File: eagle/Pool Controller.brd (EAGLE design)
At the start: 67.3 x 64.4 mm, 27 parts, among them J1 POWER_JACKPTH, J2 Temp_Pool, J3 Relay, J4 Solar_Mon, J5 Temp_Solar

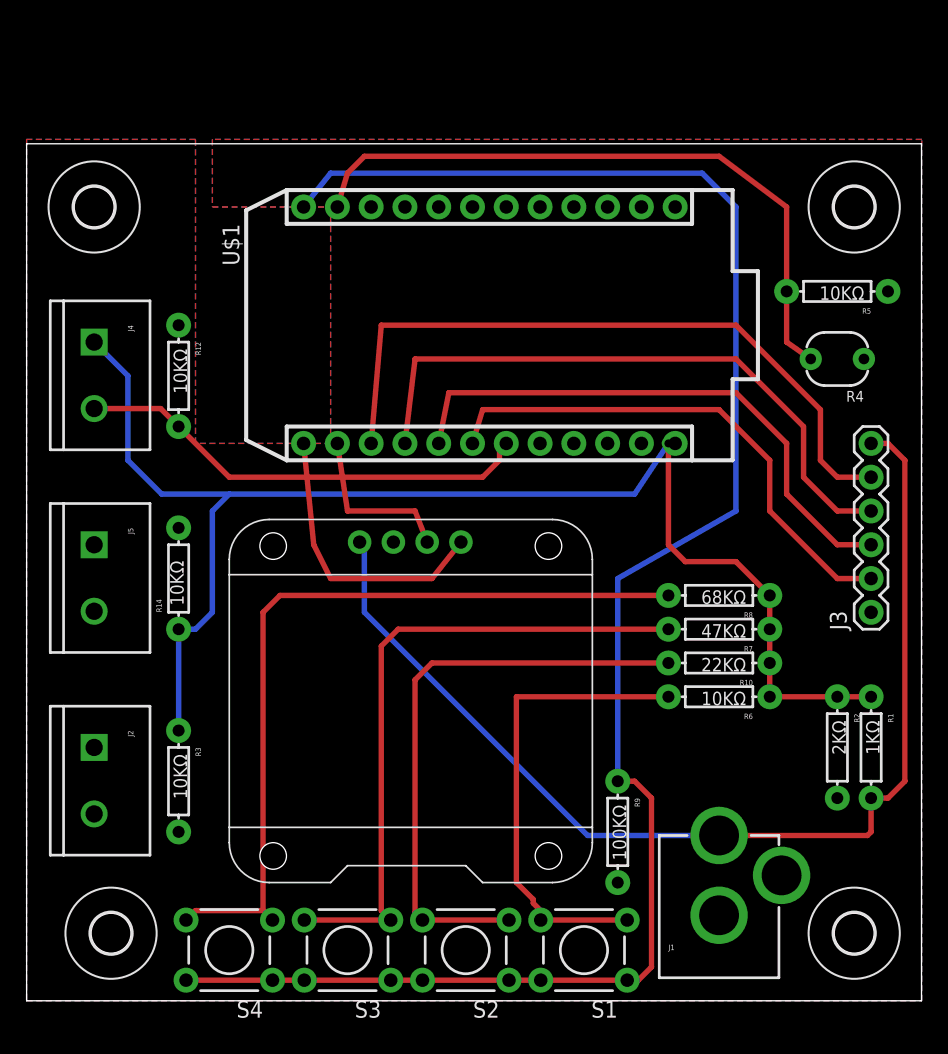
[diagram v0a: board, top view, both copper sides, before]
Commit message: Finished initial design
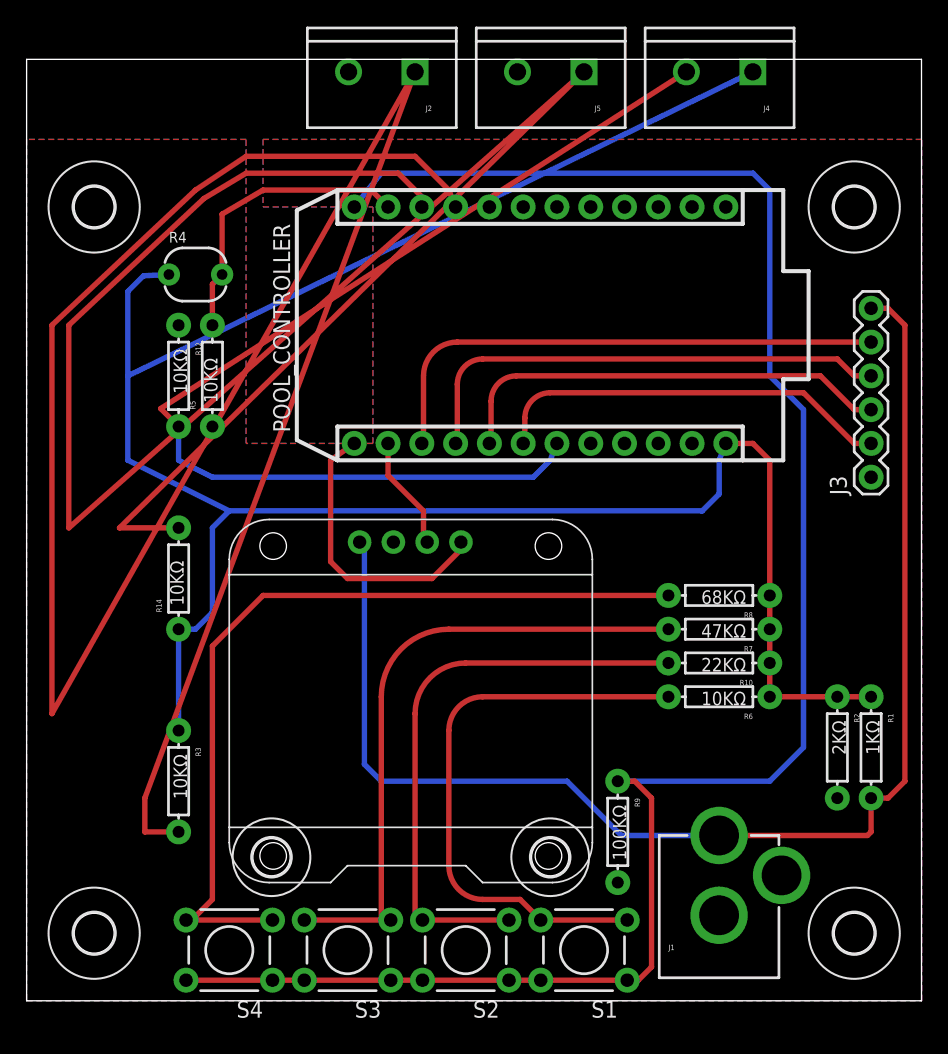
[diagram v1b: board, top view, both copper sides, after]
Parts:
- added POOL_CONTROLLER: PHOTON_WITH_HEADERS, Spark:PHOTON
- added U$7: (no value), holes:2,8
- U$1: value PHOTON_WITH_HEADERS -> (none); device Spark:PHOTON -> holes:2,8
- moved J2 56.2 mm to (27.9, 69.8), turned to 180 degrees
- moved J4 53.5 mm to (53.3, 69.8), turned to 180 degrees
- moved J5 51.2 mm to (40.6, 69.8), turned to 180 degrees
- moved U$1 50.2 mm to (17.1, 10.8), turned to 0 degrees
- moved R4 48.7 mm to (11.4, 54.6), turned to 0 degrees
- moved R5 47.4 mm to (12.7, 47.0), turned to 90 degrees
- moved J3 10.2 mm to (62.2, 39.4)
- moved U$4 1.27 mm to (3.81, 5.08)
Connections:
- removed net VCC: R4.1
- net 3.3V: now also POOL_CONTROLLER.24, R4.1; no longer U$1.24
- net GND: now also POOL_CONTROLLER.2, POOL_CONTROLLER.21; no longer U$1.2, U$1.21
- net N$1: now also POOL_CONTROLLER.15; no longer U$1.15
- net N$11: now also POOL_CONTROLLER.10; no longer U$1.10
- net N$12: now also POOL_CONTROLLER.9; no longer U$1.9
- net N$14: now also POOL_CONTROLLER.12; no longer U$1.12
- net N$2: now also POOL_CONTROLLER.16; no longer U$1.16
- net N$3: now also POOL_CONTROLLER.13; no longer U$1.13
- net N$4: now also POOL_CONTROLLER.14; no longer U$1.14
- net N$5: now also POOL_CONTROLLER.11; no longer U$1.11
- net N$6: now also POOL_CONTROLLER.17; no longer U$1.17
- net N$7: now also POOL_CONTROLLER.18; no longer U$1.18
- net N$9: now also POOL_CONTROLLER.19; no longer U$1.19
- net VBAT: now also POOL_CONTROLLER.22; no longer U$1.22
- net VIN: now also POOL_CONTROLLER.1; no longer U$1.1
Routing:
- net N$12: track 0.00 -> 185.1 mm
- net N$11: track 0.00 -> 152.7 mm
- net 3.3V: track 106.6 -> 166.4 mm, vias 1 -> 0
- net N$9: track 34.6 -> 81.5 mm
- net N$5: track 49.8 -> 22.1 mm
- net 5V: track 83.5 -> 100.3 mm
- net N$1: track 52.7 -> 39.8 mm
- net N$2: track 47.7 -> 36.9 mm
- net N$7: track 39.4 -> 30.4 mm
- net N$6: track 42.6 -> 33.6 mm
- net N$14: track 134.3 -> 142.2 mm
- net N$15: track 35.8 -> 42.8 mm
- net N$4: track 12.7 -> 8.64 mm
- net N$13: track 60.5 -> 64.0 mm
- net N$8: track 49.5 -> 47.0 mm
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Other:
- board size 67.3 x 64.4 mm -> 67.3 x 70.8 mm
